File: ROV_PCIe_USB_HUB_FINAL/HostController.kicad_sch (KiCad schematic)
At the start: 38 parts, among them U1 MX25V5126FZUI, U2 UPD720201K8-7x1-BAC-A, Y1 ABM8-24.000MHZ-B2-T

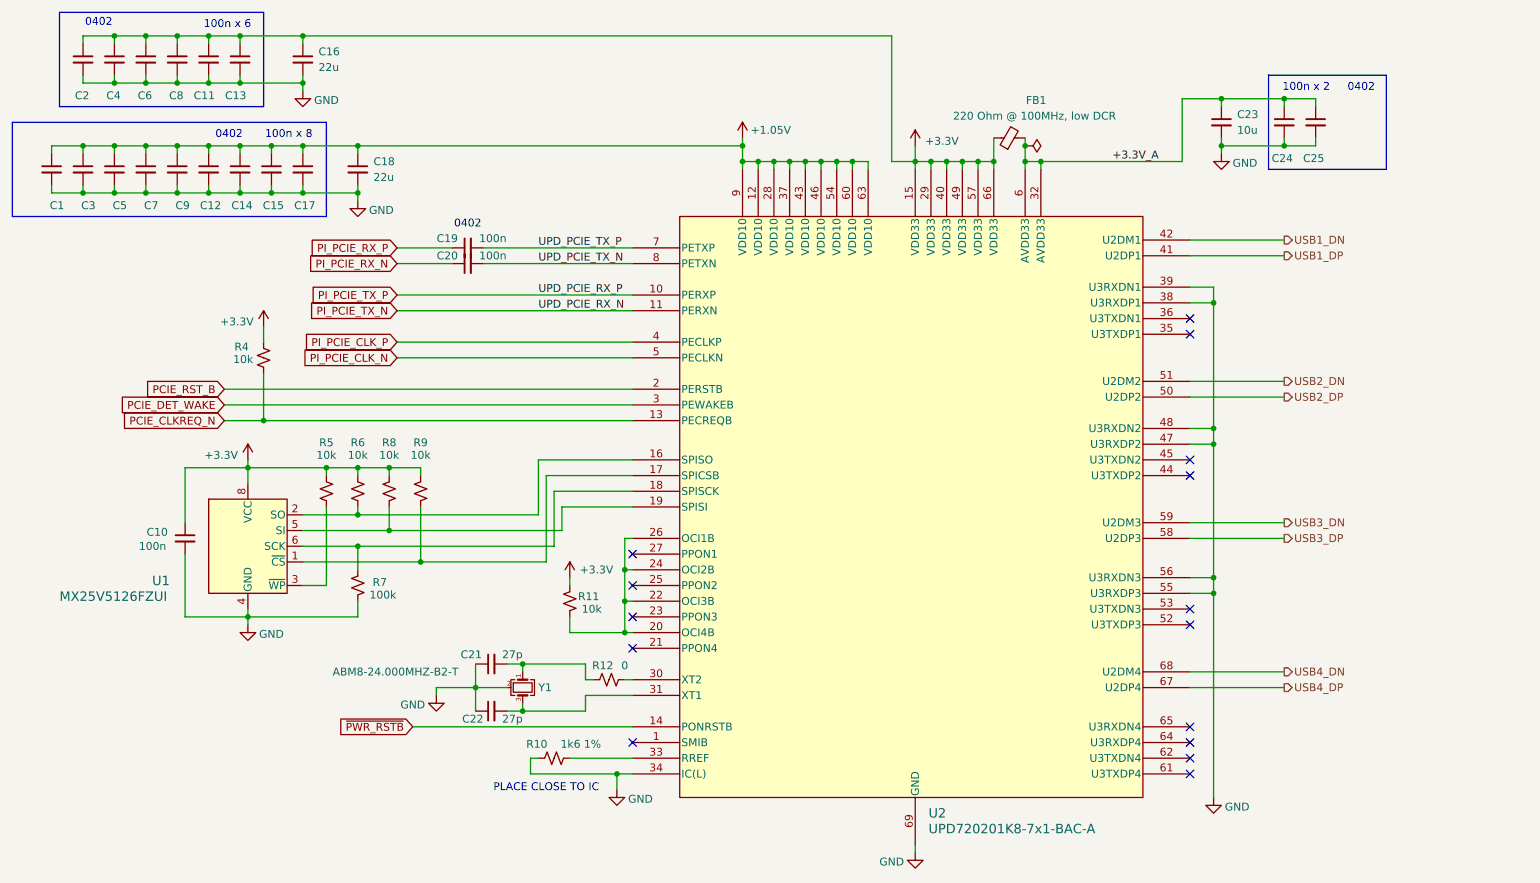
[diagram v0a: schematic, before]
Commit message: changes
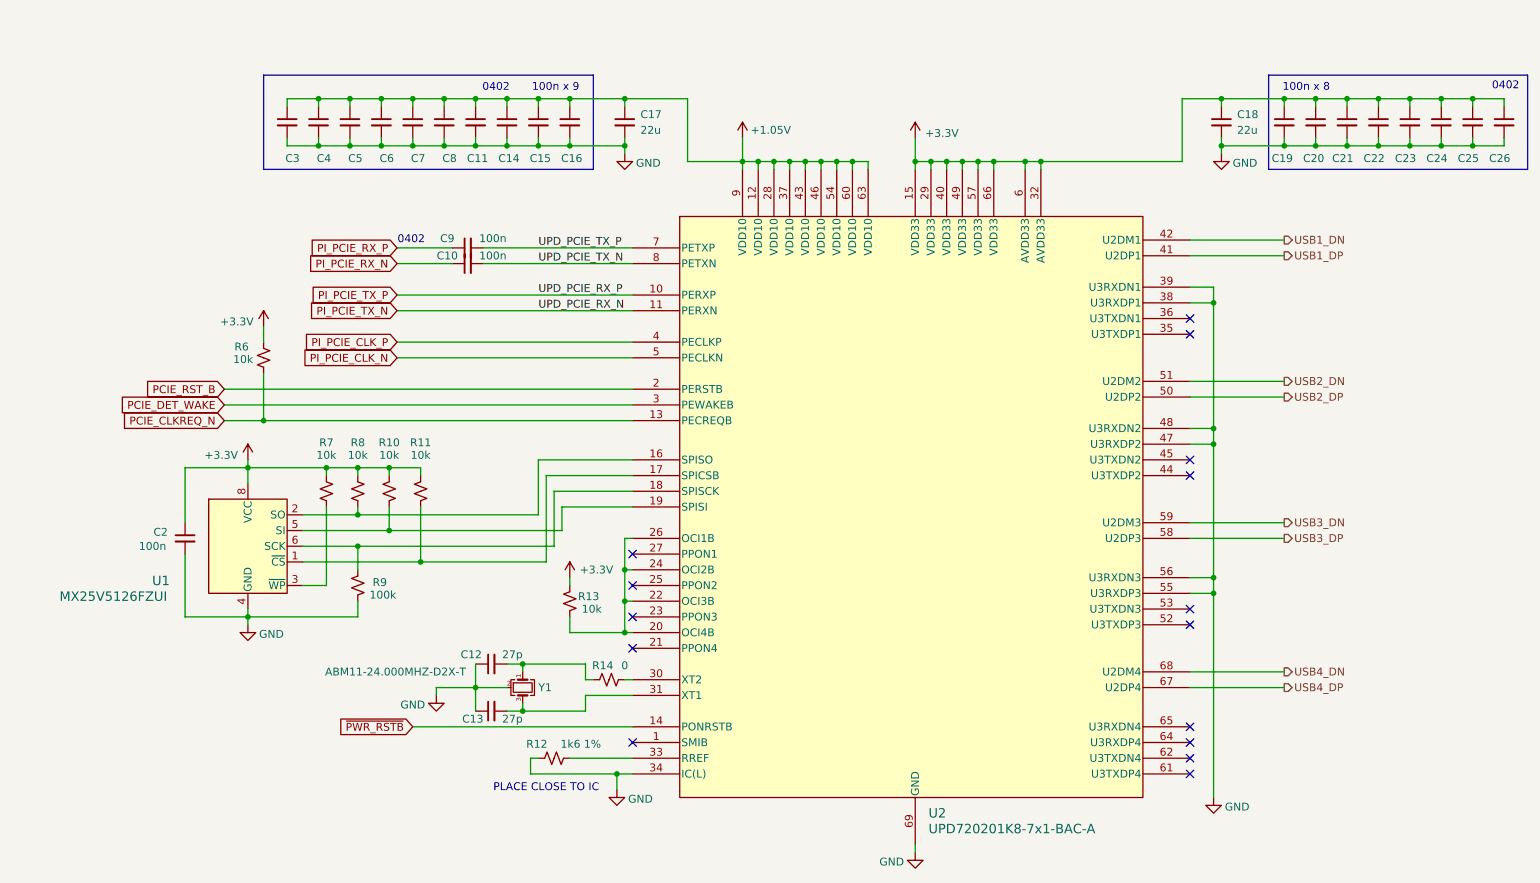
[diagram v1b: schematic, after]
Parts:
- removed C11, C13, C2, C4, C6, C8: 100n, Capacitor_SMD:C_0402_1005Metric, symbol Device:C_Small
- removed C16: 22u, Capacitor_SMD:C_1206_3216Metric, symbol Device:C_Small
- removed FB1: 220 Ohm @ 100MHz, low DCR, Inductor_SMD:L_0805_2012Metric, symbol Device:FerriteBead_Small
- added C18: 22u, Capacitor_SMD:C_1206_3216Metric, symbol Device:C_Small
- added C21, C22, C24, C25, C26, C3: 100n, Capacitor_SMD:C_0402_1005Metric, symbol Device:C_Small
- C23: value 10u -> 100n; footprint Capacitor_SMD:C_0805_2012Metric -> Capacitor_SMD:C_0402_1005Metric
- Y1: value ABM8-24.000MHZ-B2-T -> ABM11-24.000MHZ-D2X-T; footprint Crystal:Crystal_SMD_3225-4Pin_3.2x2.5mm -> Crystal:Crystal_SMD_2016-4Pin_2.0x1.6mm
- renumbered C20 to C10, C12 to C11, C21 to C12, C22 to C13, C17 to C16, C18 to C17, C24 to C19, C10 to C2, C25 to C20, C1 to C4, C3 to C5, C5 to C6, C9 to C8, C19 to C9, R8 to R10, R9 to R11, R10 to R12, R11 to R13, R12 to R14, R4 to R6, R5 to R7, R6 to R8, R7 to R9
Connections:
- net +3.3V_A is gone; now on net +3.3V: C19.1, C20.1, C23.1, U2.32 (AVDD33), U2.6 (AVDD33)
- net +1.05V: now also C3.1
- net +3.3V: now also C18.1, C21.1, C22.1, C24.1, C25.1, C26.1
- net GND: now also C18.2, C21.2, C22.2, C24.2, C25.2, C26.2, C3.2
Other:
- note added: "100n x 9"
- note removed: "100n x 2"
- note removed: "100n x 6"
- moved on the sheet: C11, C14, C15, C16, C17, C4, C5, C6, C7, C8

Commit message: work
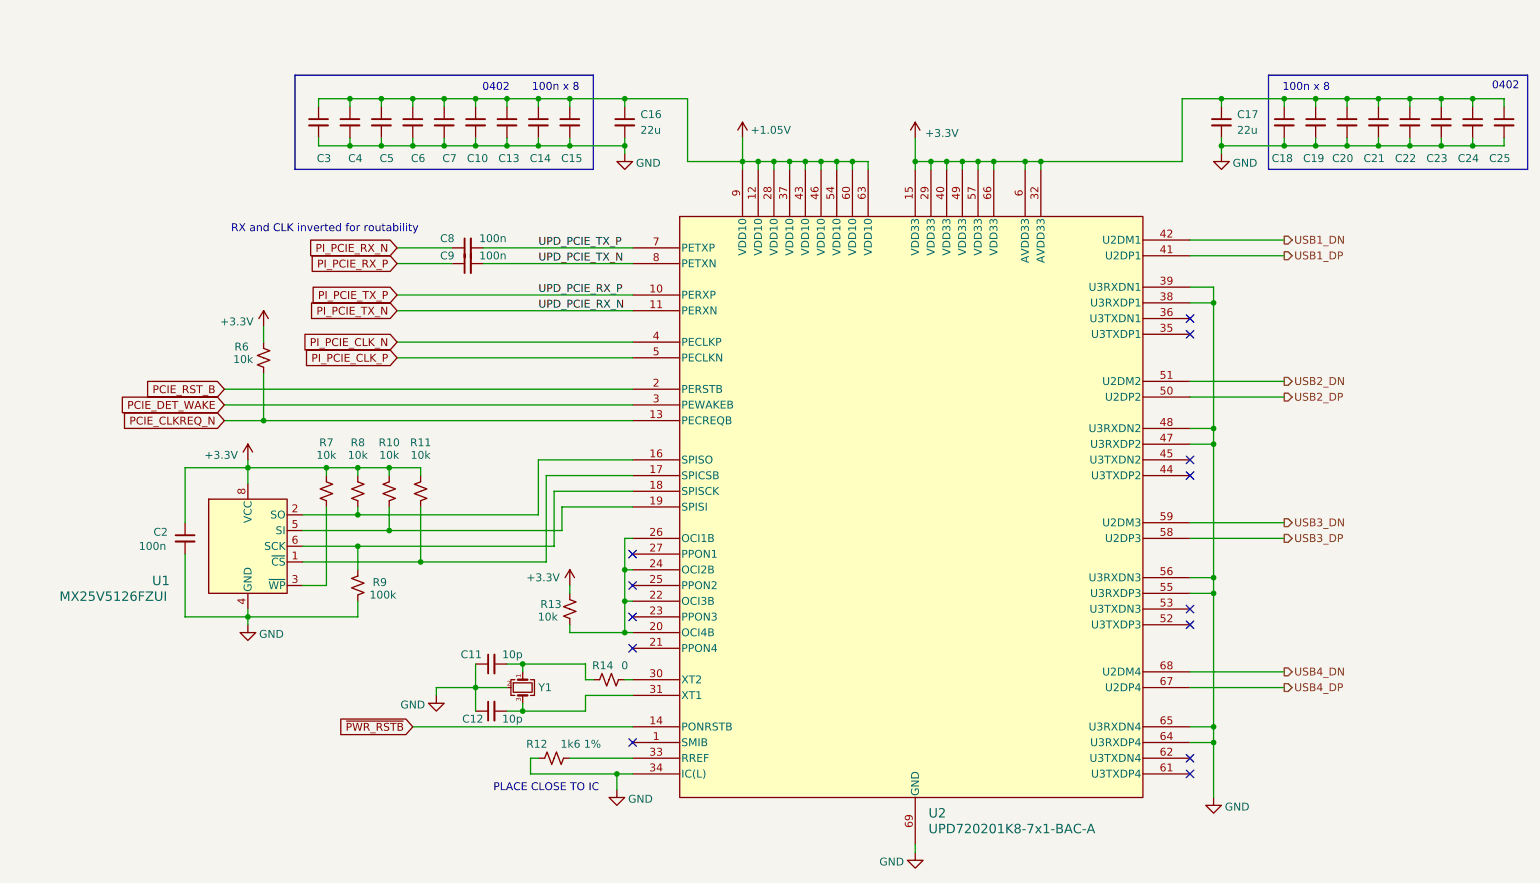
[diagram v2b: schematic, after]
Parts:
- removed C3: 100n, Capacitor_SMD:C_0402_1005Metric, symbol Device:C_Small
- C11: renamed from C12; value 27p -> 10p
- C12: renamed from C13; value 27p -> 10p
- Y1: value ABM11-24.000MHZ-D2X-T -> ECS-240-8-37B-CKY-TR
- renumbered C11 to C10, C14 to C13, C15 to C14, C16 to C15, C17 to C16, C18 to C17, C19 to C18, C20 to C19, C21 to C20, C22 to C21, C23 to C22, C24 to C23, C25 to C24, C26 to C25, C4 to C3, C5 to C4, C6 to C5, C7 to C6, C8 to C7, C9 to C8, C10 to C9
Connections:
- net GND: now also U2.64 (U3RXDP4), U2.65 (U3RXDN4)
- net PI_PCIE_CLK_N: now also U2.4 (PECLKP); no longer U2.5 (PECLKN)
- net PI_PCIE_CLK_P: now also U2.5 (PECLKN); no longer U2.4 (PECLKP)
- net PI_PCIE_RX_N: now also C8.1; no longer C9.1
- net PI_PCIE_RX_P: now also C9.1; no longer C8.1
- no-connect marks 15 -> 13
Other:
- note added: "RX and CLK inverted for routability"
- note removed: "100n x 9"
- moved on the sheet: R13

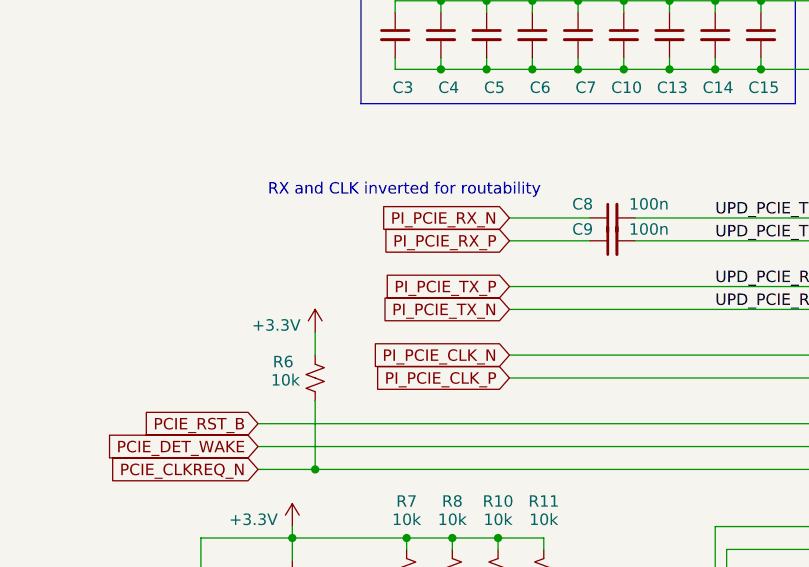
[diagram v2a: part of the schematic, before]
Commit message: reroute
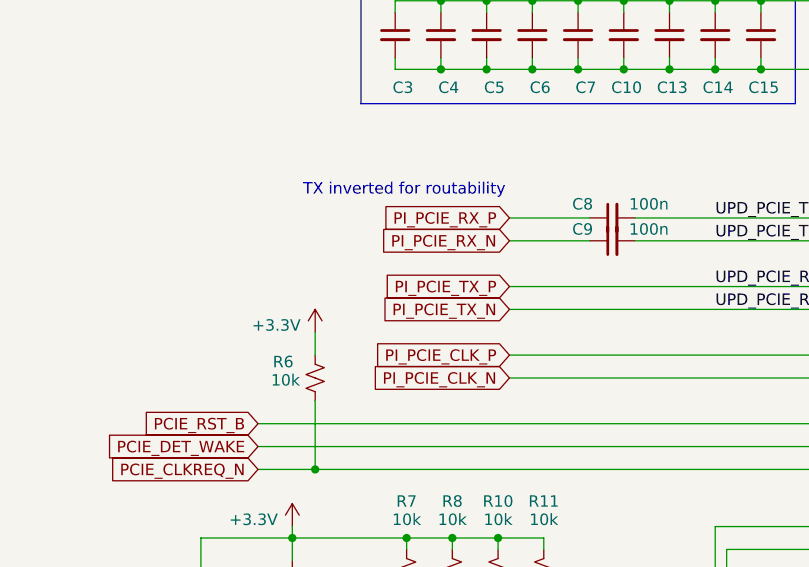
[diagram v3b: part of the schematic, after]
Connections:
- net PI_PCIE_CLK_N: now also U2.5 (PECLKN); no longer U2.4 (PECLKP)
- net PI_PCIE_CLK_P: now also U2.4 (PECLKP); no longer U2.5 (PECLKN)
- net PI_PCIE_RX_N: now also C9.1; no longer C8.1
- net PI_PCIE_RX_P: now also C8.1; no longer C9.1
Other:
- note added: "TX inverted for routability"
- note removed: "RX and CLK inverted for routability"
